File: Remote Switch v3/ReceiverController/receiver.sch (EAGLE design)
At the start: 41 parts, among them IC1 LNK304, IC2 MCP1703CB, IC3 STM8L101F2, J1 POWER_CONN_4, T1 BT136

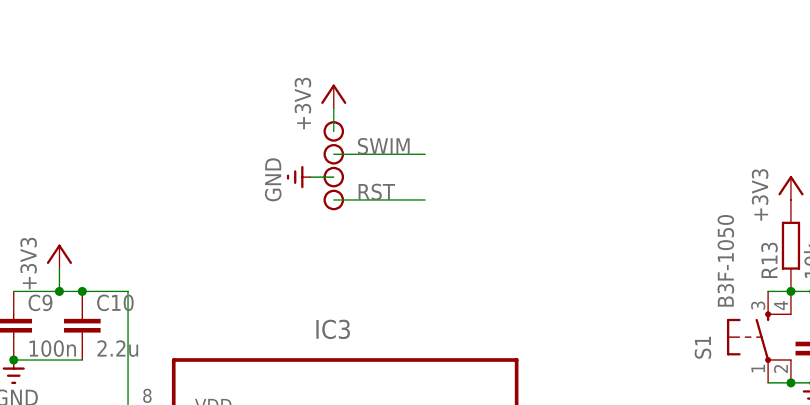
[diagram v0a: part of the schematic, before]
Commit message: PCB work
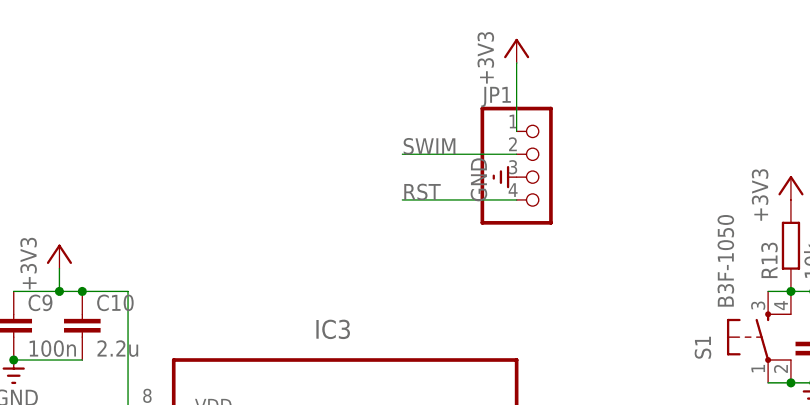
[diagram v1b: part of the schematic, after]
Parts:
- removed SIG_1, SIG_2, SIG_3, SIG_4: CON_PAD, componente_RFSwitch:CON_PAD
- added JP1: (no value), pinhead:PINHD-1X4
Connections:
- net +3V3: now also JP1.1; no longer SIG_1.P$1
- net GND: now also JP1.3; no longer SIG_3.P$1
- net RST: now also JP1.4; no longer SIG_4.P$1
- net SWIM: now also JP1.2; no longer SIG_2.P$1
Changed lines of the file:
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@@
 <part name="+3V36" library="supply1" deviceset="+3V3" device=""/>
 <part name="J1" library="CarReceiver" deviceset="POWER_CONN_4" device=""/>
-<part name="SIG_1" library="componente_RFSwitch" deviceset="CON_PAD" device=""/>
-<part name="SIG_2" library="componente_RFSwitch" deviceset="CON_PAD" device=""/>
-<part name="SIG_3" library="componente_RFSwitch" deviceset="CON_PAD" device=""/>
-<part name="SIG_4" library="componente_RFSwitch" deviceset="CON_PAD" device=""/>
 <part name="+3V35" library="supply1" deviceset="+3V3" device=""/>
 <part name="GND15" library="supply" deviceset="GND" device=""/>
@@
 <part name="C13" library="resistor" deviceset="C-EU" device="C0603K" value="100n"/>
 <part name="GND17" library="supply" deviceset="GND" device=""/>
+<part name="JP1" library="pinhead" deviceset="PINHD-1X4" device=""/>
 </parts>
 <sheets>
@@
 <instance part="+3V36" gate="G$1" x="238.76" y="157.48"/>
 <instance part="J1" gate="G$1" x="17.78" y="129.54"/>
-<instance part="SIG_1" gate="G$1" x="187.96" y="162.56"/>
-<instance part="SIG_2" gate="G$1" x="187.96" y="160.02"/>
-<instance part="SIG_3" gate="G$1" x="187.96" y="157.48"/>
-<instance part="SIG_4" gate="G$1" x="187.96" y="154.94"/>
-<instance part="+3V35" gate="G$1" x="187.96" y="167.64"/>
-<instance part="GND15" gate="1" x="182.88" y="157.48" rot="R270"/>
+<instance part="+3V35" gate="G$1" x="208.28" y="172.72"/>
+<instance part="GND15" gate="1" x="205.74" y="157.48" rot="R270"/>
 <instance part="LED1" gate="G$1" x="53.34" y="162.56" rot="R270"/>
 <instance part="R1" gate="G$1" x="25.4" y="33.02" rot="R180"/>
@@
 <instance part="C13" gate="G$1" x="157.48" y="50.8"/>
 <instance part="GND17" gate="1" x="157.48" y="43.18"/>
+<instance part="JP1" gate="A" x="210.82" y="157.48"/>
 </instances>
 <busses>
@@
 </segment>
 <segment>
-<pinref part="SIG_4" gate="G$1" pin="P$1"/>
-<wire x1="187.96" y1="154.94" x2="198.12" y2="154.94" width="0.1524" layer="91"/>
-<label x="190.5" y="154.94" size="1.778" layer="95"/>
+<pinref part="JP1" gate="A" pin="4"/>
+<wire x1="208.28" y1="154.94" x2="195.58" y2="154.94" width="0.1524" layer="91"/>
+<label x="195.58" y="154.94" size="1.778" layer="95"/>
 </segment>
 </net>
@@
 <junction x="152.4" y="137.16"/>
 <pinref part="C10" gate="G$1" pin="2"/>
-</segment>
-<segment>
-<pinref part="SIG_3" gate="G$1" pin="P$1"/>
-<pinref part="GND15" gate="1" pin="GND"/>
-<wire x1="185.42" y1="157.48" x2="187.96" y2="157.48" width="0.1524" layer="91"/>
 </segment>
 <segment>
@@
 <pinref part="C13" gate="G$1" pin="2"/>
 <pinref part="GND17" gate="1" pin="GND"/>
+</segment>
+<segment>
+<pinref part="JP1" gate="A" pin="3"/>
+<pinref part="GND15" gate="1" pin="GND"/>
 </segment>
 </net>
@@
 </segment>
 <segment>
-<pinref part="SIG_2" gate="G$1" pin="P$1"/>
-<wire x1="187.96" y1="160.02" x2="198.12" y2="160.02" width="0.1524" layer="91"/>
-<label x="190.5" y="160.02" size="1.778" layer="95"/>
+<pinref part="JP1" gate="A" pin="2"/>
+<wire x1="208.28" y1="160.02" x2="195.58" y2="160.02" width="0.1524" layer="91"/>
+<label x="195.58" y="160.02" size="1.778" layer="95"/>
 </segment>
 </net>
@@
 </segment>
 <segment>
-<pinref part="SIG_1" gate="G$1" pin="P$1"/>
-<pinref part="+3V35" gate="G$1" pin="+3V3"/>
-<wire x1="187.96" y1="165.1" x2="187.96" y2="162.56" width="0.1524" layer="91"/>
-</segment>
-<segment>
 <pinref part="IC2" gate="G$1" pin="VO"/>
 <pinref part="C11" gate="G$1" pin="1"/>
@@
 <wire x1="25.4" y1="93.98" x2="15.24" y2="93.98" width="0.1524" layer="91"/>
 </segment>
-</net>
+<segment>
+<pinref part="+3V35" gate="G$1" pin="+3V3"/>
+<pinref part="JP1" gate="A" pin="1"/>
+<wire x1="208.28" y1="170.18" x2="208.28" y2="162.56" width="0.1524" layer="91"/>
+</segment>
+</net>

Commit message: PCB work
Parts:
- C4: device resistor:C-EUC0805K -> resistor:C-EUC0603K
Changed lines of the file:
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@@
 <grid distance="0.1" unitdist="inch" unit="inch" style="lines" multiple="1" display="no" altdistance="0.01" altunitdist="inch" altunit="inch"/>
 <layers>
-<layer number="1" name="Top" color="4" fill="1" visible="no" active="no"/>
-<layer number="16" name="Bottom" color="1" fill="1" visible="no" active="no"/>
-<layer number="17" name="Pads" color="2" fill="1" visible="no" active="no"/>
-<layer number="18" name="Vias" color="2" fill="1" visible="no" active="no"/>
-<layer number="19" name="Unrouted" color="6" fill="1" visible="no" active="no"/>
-<layer number="20" name="Dimension" color="15" fill="1" visible="no" active="no"/>
-<layer number="21" name="tPlace" color="7" fill="1" visible="no" active="no"/>
-<layer number="22" name="bPlace" color="7" fill="1" visible="no" active="no"/>
-<layer number="23" name="tOrigins" color="15" fill="1" visible="no" active="no"/>
-<layer number="24" name="bOrigins" color="15" fill="1" visible="no" active="no"/>
-<layer number="25" name="tNames" color="7" fill="1" visible="no" active="no"/>
-<layer number="26" name="bNames" color="7" fill="1" visible="no" active="no"/>
-<layer number="27" name="tValues" color="7" fill="1" visible="no" active="no"/>
-<layer number="28" name="bValues" color="7" fill="1" visible="no" active="no"/>
+<layer number="1" name="Top" color="4" fill="1" visible="yes" active="no"/>
+<layer number="16" name="Bottom" color="1" fill="1" visible="yes" active="no"/>
+<layer number="17" name="Pads" color="2" fill="1" visible="yes" active="no"/>
+<layer number="18" name="Vias" color="2" fill="1" visible="yes" active="no"/>
+<layer number="19" name="Unrouted" color="6" fill="1" visible="yes" active="no"/>
+<layer number="20" name="Dimension" color="15" fill="1" visible="yes" active="no"/>
+<layer number="21" name="tPlace" color="7" fill="1" visible="yes" active="no"/>
+<layer number="22" name="bPlace" color="7" fill="1" visible="yes" active="no"/>
+<layer number="23" name="tOrigins" color="15" fill="1" visible="yes" active="no"/>
+<layer number="24" name="bOrigins" color="15" fill="1" visible="yes" active="no"/>
+<layer number="25" name="tNames" color="7" fill="1" visible="yes" active="no"/>
+<layer number="26" name="bNames" color="7" fill="1" visible="yes" active="no"/>
+<layer number="27" name="tValues" color="7" fill="1" visible="yes" active="no"/>
+<layer number="28" name="bValues" color="7" fill="1" visible="yes" active="no"/>
 <layer number="29" name="tStop" color="7" fill="3" visible="no" active="no"/>
 <layer number="30" name="bStop" color="7" fill="6" visible="no" active="no"/>
@@
 <layer number="35" name="tGlue" color="7" fill="4" visible="no" active="no"/>
 <layer number="36" name="bGlue" color="7" fill="5" visible="no" active="no"/>
-<layer number="37" name="tTest" color="7" fill="1" visible="no" active="no"/>
-<layer number="38" name="bTest" color="7" fill="1" visible="no" active="no"/>
+<layer number="37" name="tTest" color="7" fill="1" visible="yes" active="no"/>
+<layer number="38" name="bTest" color="7" fill="1" visible="yes" active="no"/>
 <layer number="39" name="tKeepout" color="4" fill="11" visible="no" active="no"/>
 <layer number="40" name="bKeepout" color="1" fill="11" visible="no" active="no"/>
@@
 <layer number="44" name="Drills" color="7" fill="1" visible="no" active="no"/>
 <layer number="45" name="Holes" color="7" fill="1" visible="no" active="no"/>
-<layer number="46" name="Milling" color="3" fill="1" visible="no" active="no"/>
-<layer number="47" name="Measures" color="7" fill="1" visible="no" active="no"/>
-<layer number="48" name="Document" color="7" fill="1" visible="no" active="no"/>
-<layer number="49" name="Reference" color="7" fill="1" visible="no" active="no"/>
-<layer number="50" name="dxf" color="7" fill="1" visible="no" active="no"/>
-<layer number="51" name="tDocu" color="7" fill="1" visible="no" active="no"/>
-<layer number="52" name="bDocu" color="7" fill="1" visible="no" active="no"/>
-<layer number="53" name="tGND_GNDA" color="7" fill="9" visible="no" active="no"/>
-<layer number="54" name="bGND_GNDA" color="1" fill="9" visible="no" active="no"/>
-<layer number="56" name="wert" color="7" fill="1" visible="no" active="no"/>
+<layer number="46" name="Milling" color="3" fill="1" visible="yes" active="no"/>
+<layer number="47" name="Measures" color="7" fill="1" visible="yes" active="no"/>
+<layer number="48" name="Document" color="7" fill="1" visible="yes" active="no"/>
+<layer number="49" name="Reference" color="7" fill="1" visible="yes" active="no"/>
+<layer number="50" name="dxf" color="7" fill="1" visible="yes" active="no"/>
+<layer number="51" name="tDocu" color="7" fill="1" visible="yes" active="no"/>
+<layer number="52" name="bDocu" color="7" fill="1" visible="yes" active="no"/>
+<layer number="53" name="tGND_GNDA" color="7" fill="9" visible="yes" active="no"/>
+<layer number="54" name="bGND_GNDA" color="1" fill="9" visible="yes" active="no"/>
+<layer number="56" name="wert" color="7" fill="1" visible="yes" active="no"/>
 <layer number="90" name="Modules" color="5" fill="1" visible="no" active="no"/>
 <layer number="91" name="Nets" color="2" fill="1" visible="yes" active="yes"/>
@@
 <part name="B1" library="rectifier" deviceset="B*S" device="" technology="05"/>
 <part name="C3" library="resistor" deviceset="CPOL-EU" device="E5-10.5" value="4.7u"/>
-<part name="C4" library="resistor" deviceset="C-EU" device="C0805K" value="100n"/>
+<part name="C4" library="resistor" deviceset="C-EU" device="C0603K" value="100n"/>
 <part name="C6" library="resistor" deviceset="CPOL-EU" device="D" value="100u"/>
 <part name="+3V33" library="supply1" deviceset="+3V3" device=""/>
